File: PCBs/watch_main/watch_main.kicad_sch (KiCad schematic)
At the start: 0 parts

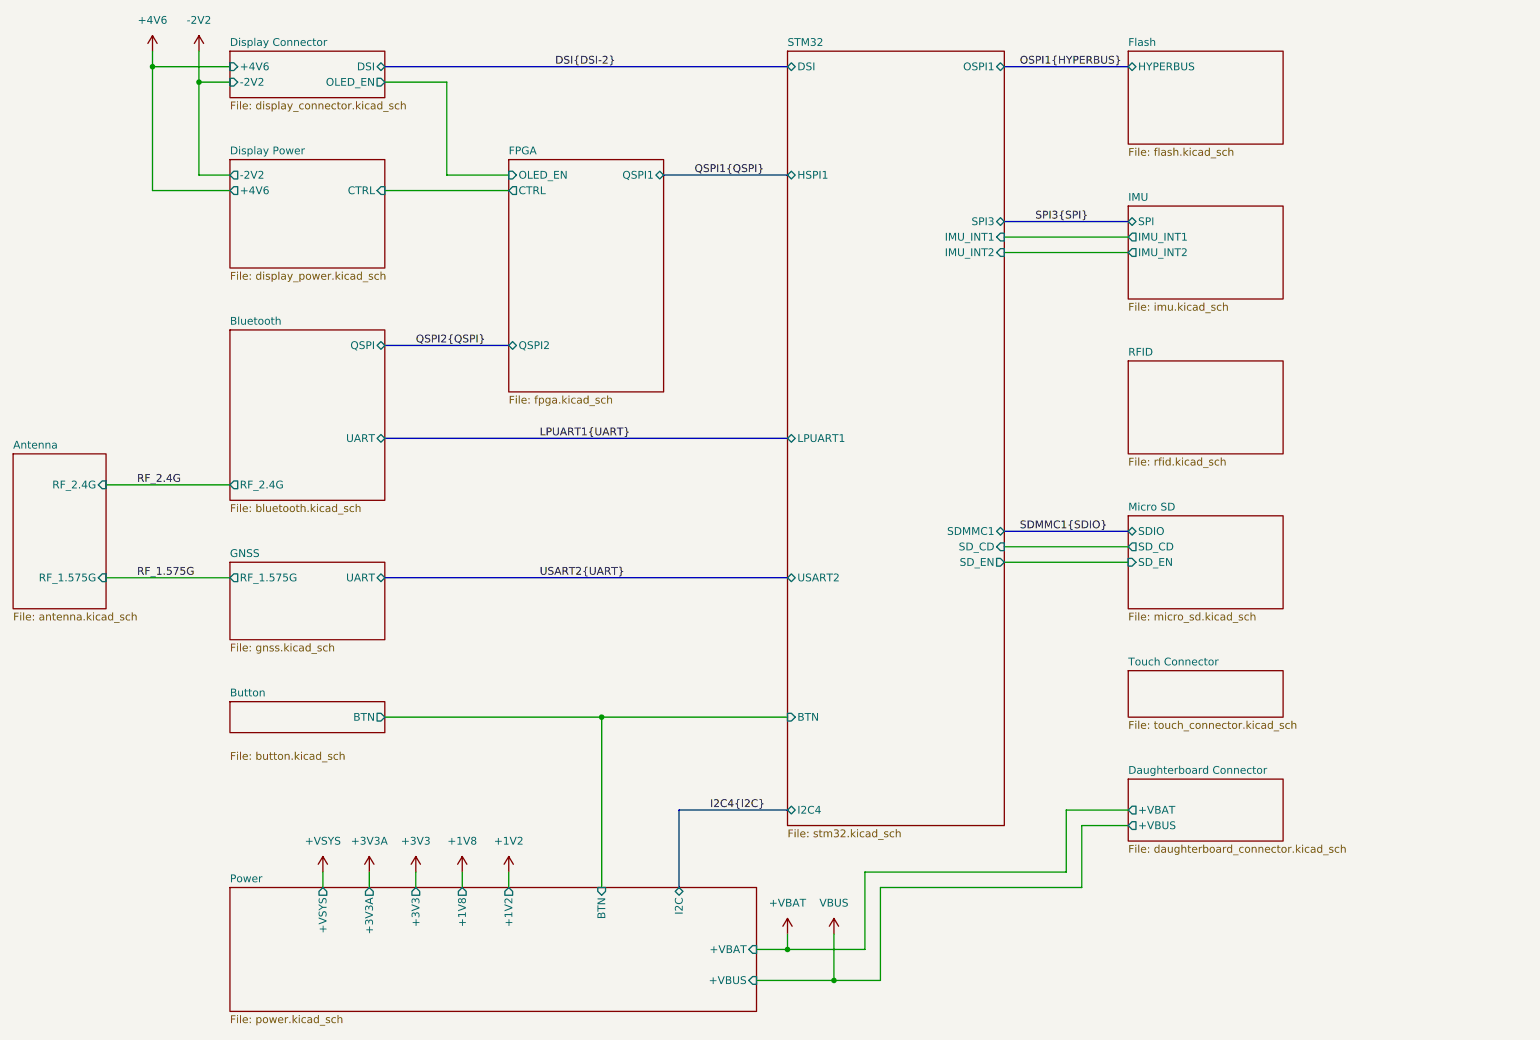
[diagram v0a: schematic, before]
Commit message: More PCB progress
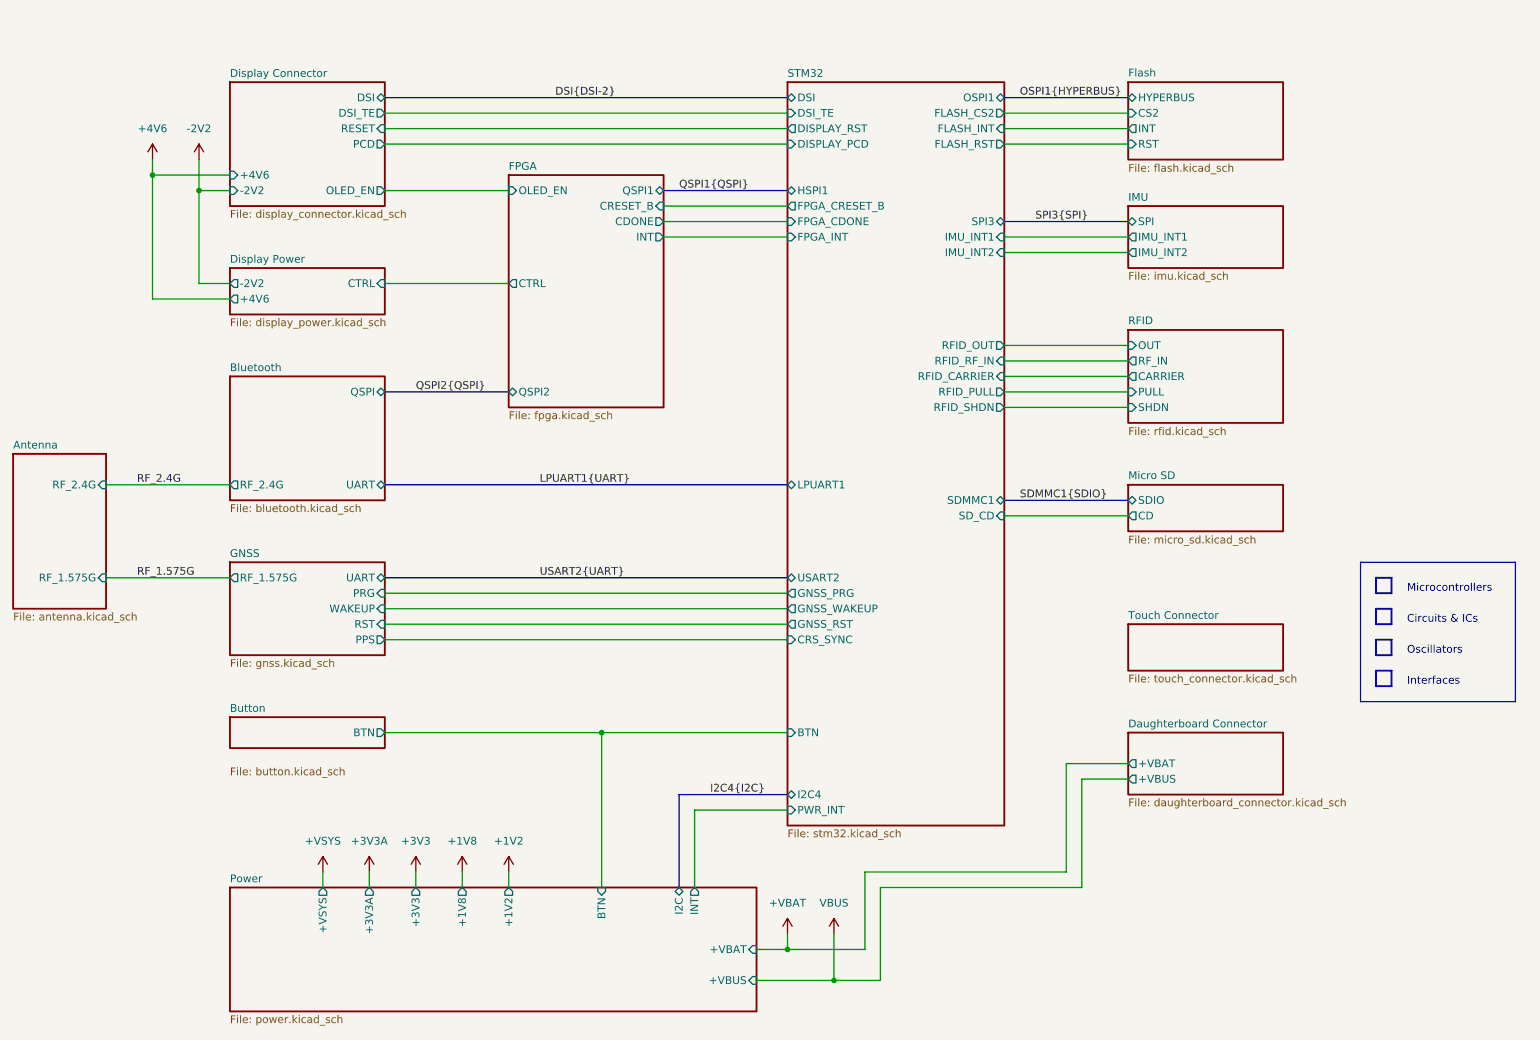
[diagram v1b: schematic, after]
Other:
- sheet Display Connector ports: added DSI_TE, PCD, RESET; removed none
- sheet FPGA ports: added CDONE, CRESET_B, INT; removed none
- sheet Flash ports: added CS2, INT, RST; removed none
- sheet GNSS ports: added PPS, PRG, RST, WAKEUP; removed none
- sheet Micro SD ports: added CD; removed SD_CD, SD_EN
- sheet Power ports: added INT; removed none
- sheet RFID ports: added CARRIER, OUT, PULL, RF_IN, SHDN; removed none
- sheet STM32 ports: added CRS_SYNC, DISPLAY_PCD, DISPLAY_RST, DSI_TE, FLASH_CS2, FLASH_INT, FLASH_RST, FPGA_CDONE, FPGA_CRESET_B, FPGA_INT, GNSS_PRG, GNSS_RST, GNSS_WAKEUP, PWR_INT, RFID_CARRIER, RFID_OUT, RFID_PULL, RFID_RF_IN, RFID_SHDN; removed SD_EN
- note added: "Circuits & ICs"
- note added: "Interfaces"
- note added: "Microcontrollers"
- note added: "Oscillators"
